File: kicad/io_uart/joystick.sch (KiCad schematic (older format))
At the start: 17 parts, among them U2 7400, U3 74LS244, U4 74125

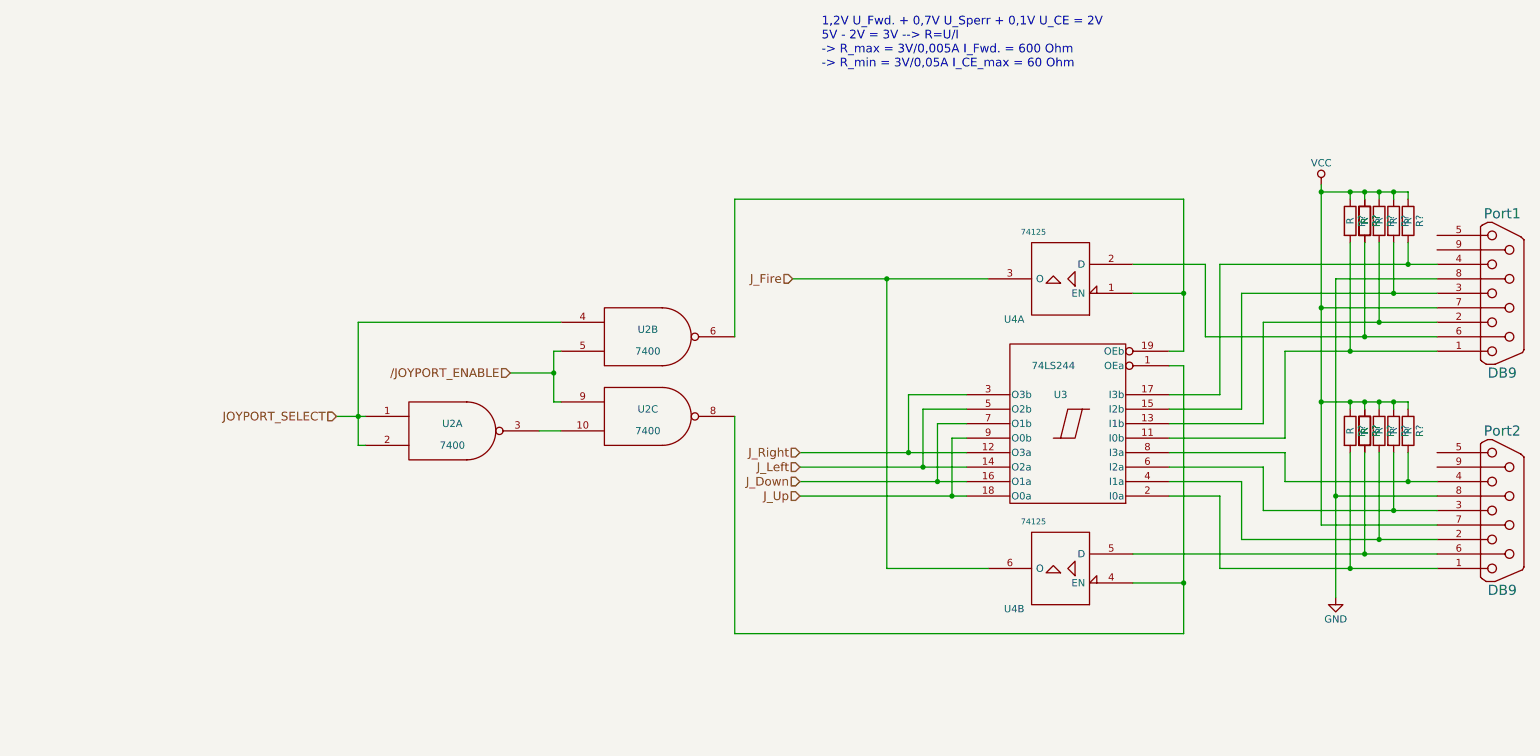
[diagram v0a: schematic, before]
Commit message: xmodem
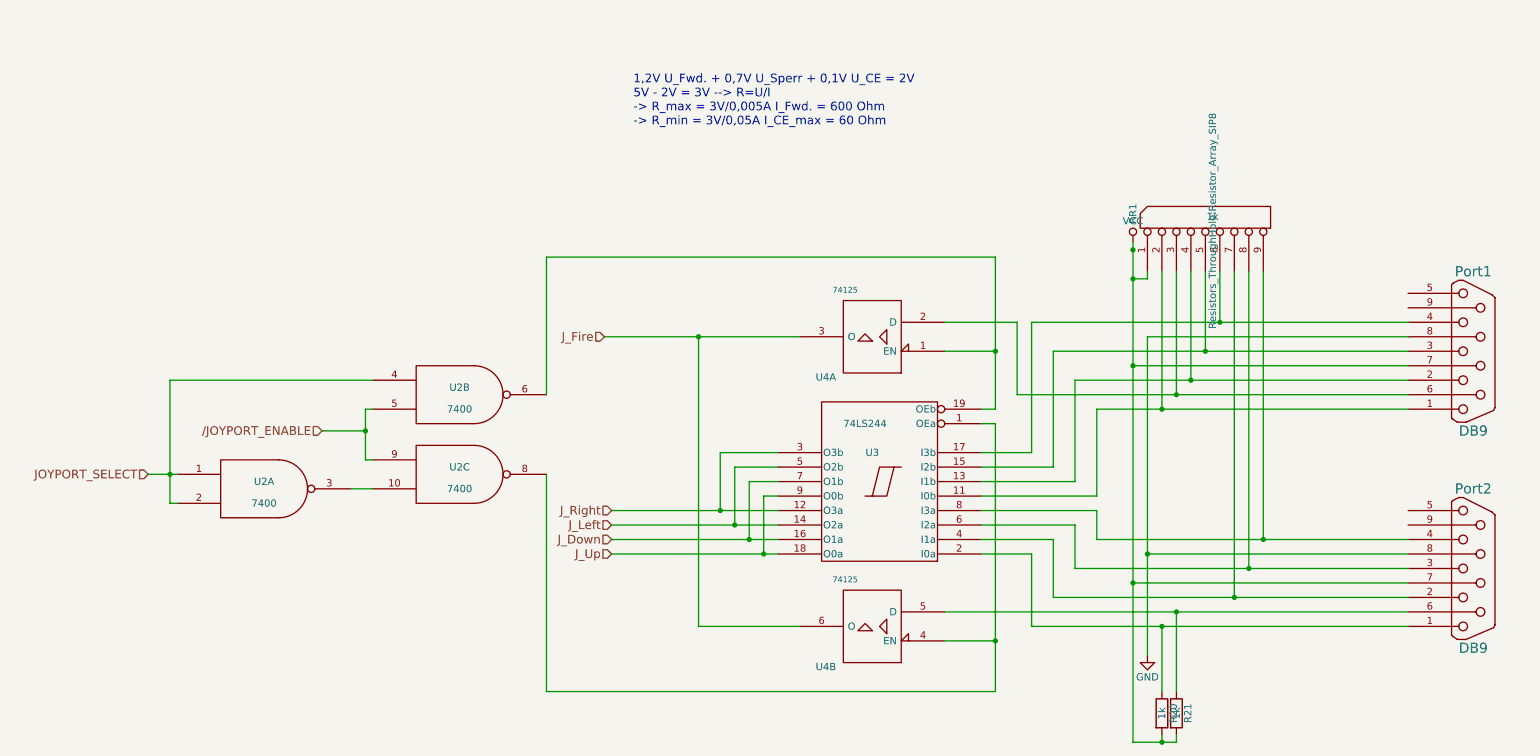
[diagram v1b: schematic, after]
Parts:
- removed R? (x12): R, symbol R
- added R20, R21: 1k, Discret:R3-LARGE_PADS, symbol R
- added RR1: 1k, Resistors_ThroughHole:Resistor_Array_SIP8, symbol RR8
- U2: footprint (none) -> Housings_DIP:DIP-14_W7.62mm_LongPads
- U3: footprint (none) -> Housings_DIP:DIP-20_W7.62mm_LongPads
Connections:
- net VCC: now also R20.2, R21.2, RR1.1 (COM)
- net at Port1.1, U3.11 (I0b): now also RR1.2
- net at Port1.2, U3.13 (I1b): now also RR1.4
- net at Port1.3, U3.15 (I2b): now also RR1.5
- net at Port1.4, U3.17 (I3b): now also RR1.6
- net at Port1.6 (P6), U4.2 (D): now also RR1.3
- net at Port2.1, U3.2 (I0a): now also R20.1
- net at Port2.2, U3.4 (I1a): now also RR1.7
- net at Port2.3, U3.6 (I2a): now also RR1.8
- net at Port2.4, U3.8 (I3a): now also RR1.9
- net at Port2.6 (P6), U4.5 (D): now also R21.1
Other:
- moved on the sheet: Port1, Port2, U2A, U2B, U2C, U3, U4A, U4B
